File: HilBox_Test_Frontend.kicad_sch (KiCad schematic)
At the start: 21 parts, among them SW1 SW_DIP_x06

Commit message: Schematic design at finish
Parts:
- D12: footprint Relays:RELAY_G6K-2F_DC5 -> LED_SMD:LED_RGB_5050-6
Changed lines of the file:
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@@
 			)
 		)
-		(property "Footprint" "Relays:RELAY_G6K-2F_DC5"
+		(property "Footprint" "LED_SMD:LED_RGB_5050-6"
 			(at 194.31 85.09 0)
 			(effects

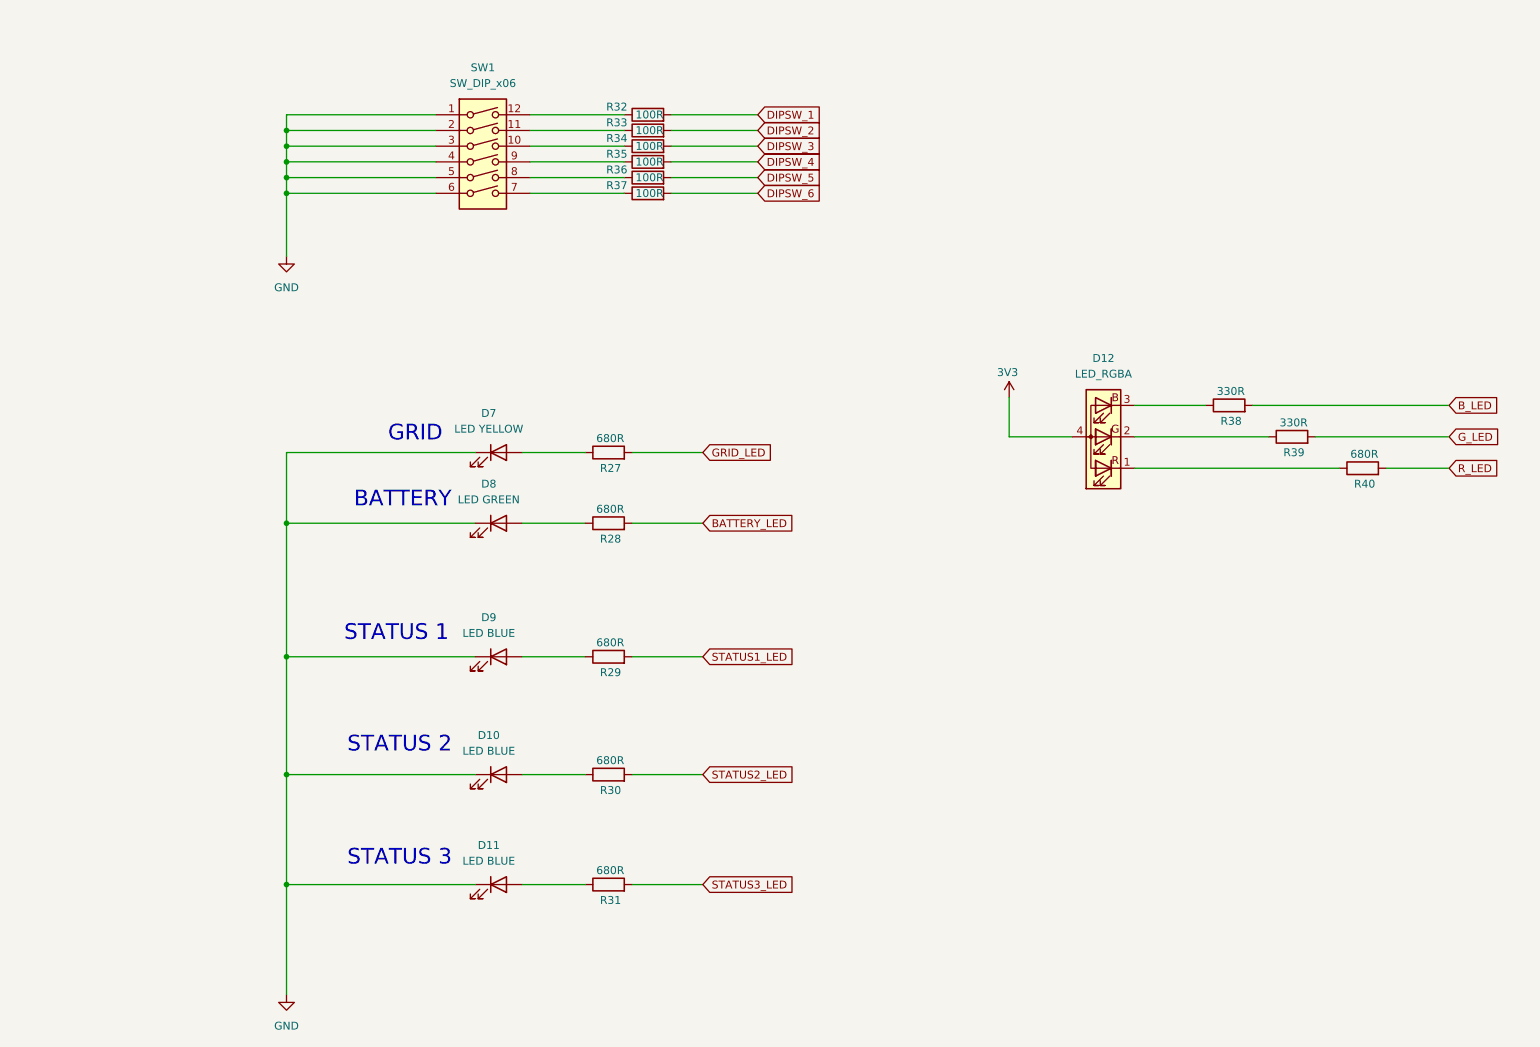
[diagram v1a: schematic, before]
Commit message: Layout 90% done
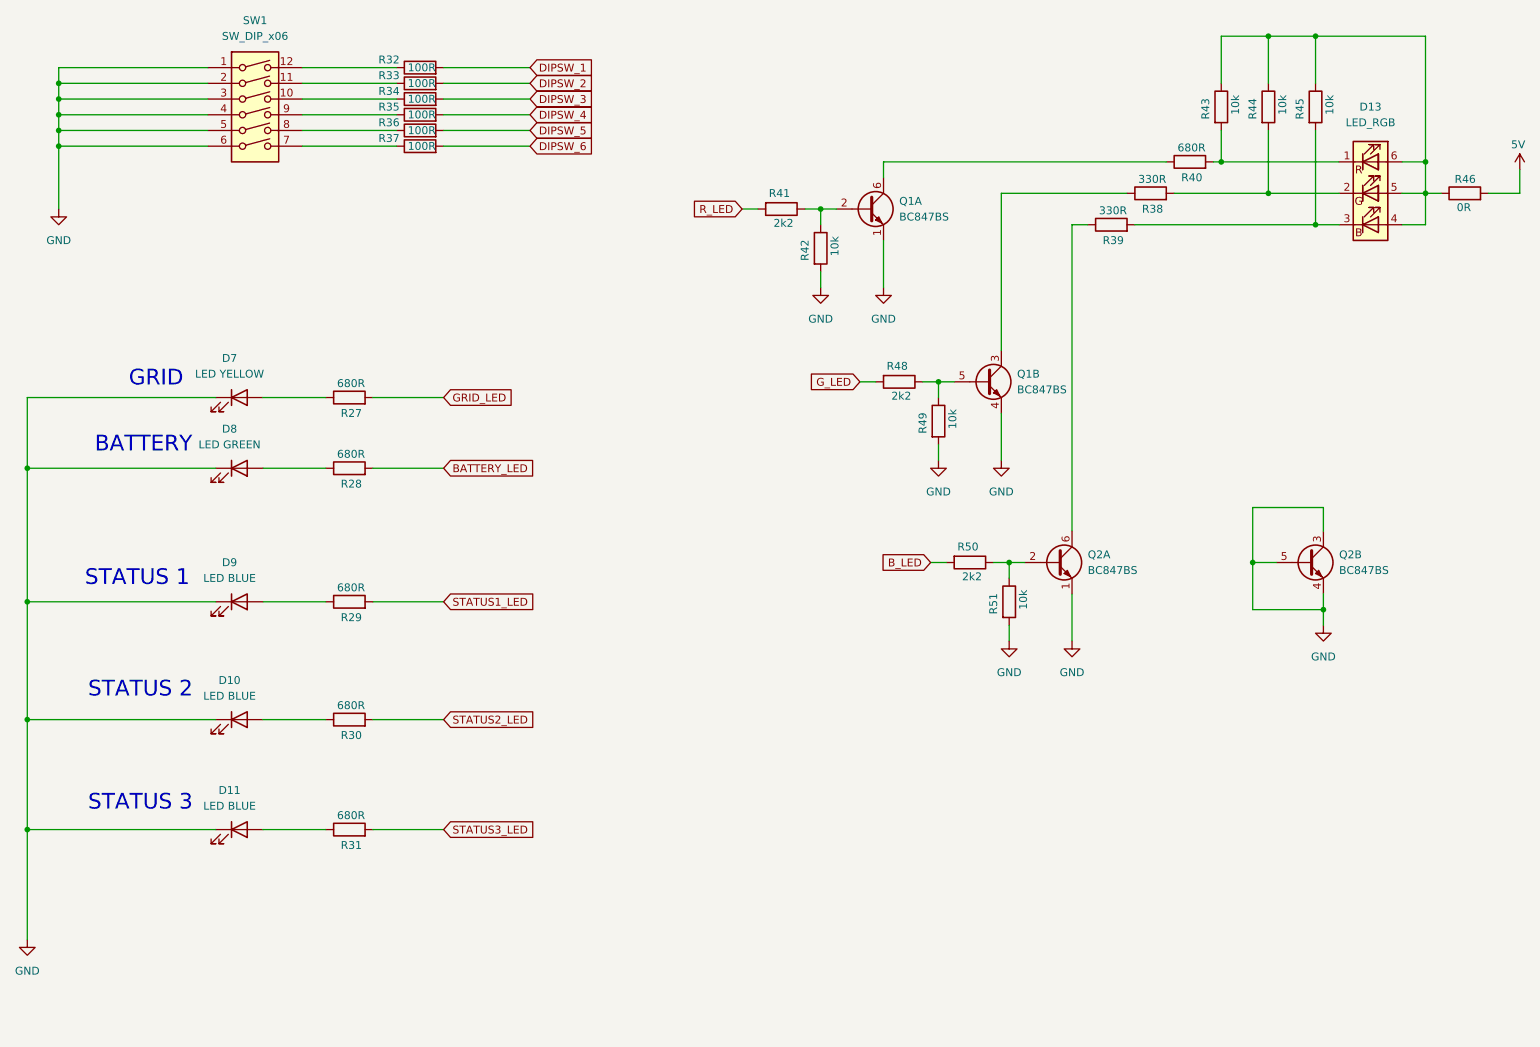
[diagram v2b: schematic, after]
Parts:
- removed D12: LED_RGBA, LED_SMD:LED_RGB_5050-6, symbol Device:LED_RGBA
- added D13: LED_RGB, LED_SMD:LED_RGB_5050-6, symbol Device:LED_RGB
- added Q1, Q2: BC847BS, Package_TO_SOT_SMD:SOT-363_SC-70-6, symbol Transistor_BJT:BC847BS
- added R41, R48, R50: 2k2, Resistor_SMD:R_0603_1608Metric, symbol Device:R
- added R42, R43, R44, R45, R49, R51: 10k, Resistor_SMD:R_0603_1608Metric, symbol Device:R
- added R46: 0R, Resistor_SMD:R_0603_1608Metric, symbol Device:R
- R38, R39: footprint Resistor_SMD:R_0603_1608Metric -> Resistor_SMD:R_1206_3216Metric; JLC_PN C12246 -> C25374
- R40: footprint Resistor_SMD:R_0603_1608Metric -> Resistor_SMD:R_1206_3216Metric; JLC_PN C25177 -> C17975
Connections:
- net B_LED: now also R50.2; no longer R38.2
- net GND: now also Q1.1 (E1), Q1.4 (E2), Q2.1 (E1), Q2.3 (C2), Q2.4 (E2), Q2.5 (B2), R42.2, R49.2, R51.2
- net G_LED: now also R48.2; no longer R39.2
- net R_LED: now also R41.2; no longer R40.2
- net at R40.1: now also Q1.6 (C1)
- net at R39.1: now also Q2.6 (C1)
- net at R38.1: now also Q1.3 (C2)
- new net: Q2.2 (B1), R50.1, R51.1
- new net: D13.4 (BA), D13.5 (GA), D13.6 (RA), R43.1, R44.1, R45.1, R46.1
- new net: D13.1 (RK), R40.2, R43.2
- new net: Q1.2 (B1), R41.1, R42.1
- new net: Q1.5 (B2), R48.1, R49.1
- new net: D13.3 (BK), R39.2, R45.2
- new net: D13.2 (GK), R38.2, R44.2
- new net 5V: R46.2
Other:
- moved on the sheet: D10, D11, D7, D8, D9, R27, R28, R29, R30, R31, R32, R33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
